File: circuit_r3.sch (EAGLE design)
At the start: 25 parts, among them IC1 7805DT, U1 MCP4725, U2 MB85RC256VPF-G-JNERE2, U4 ATMEGA328P_VQFNVQFN, Y1 16MHz

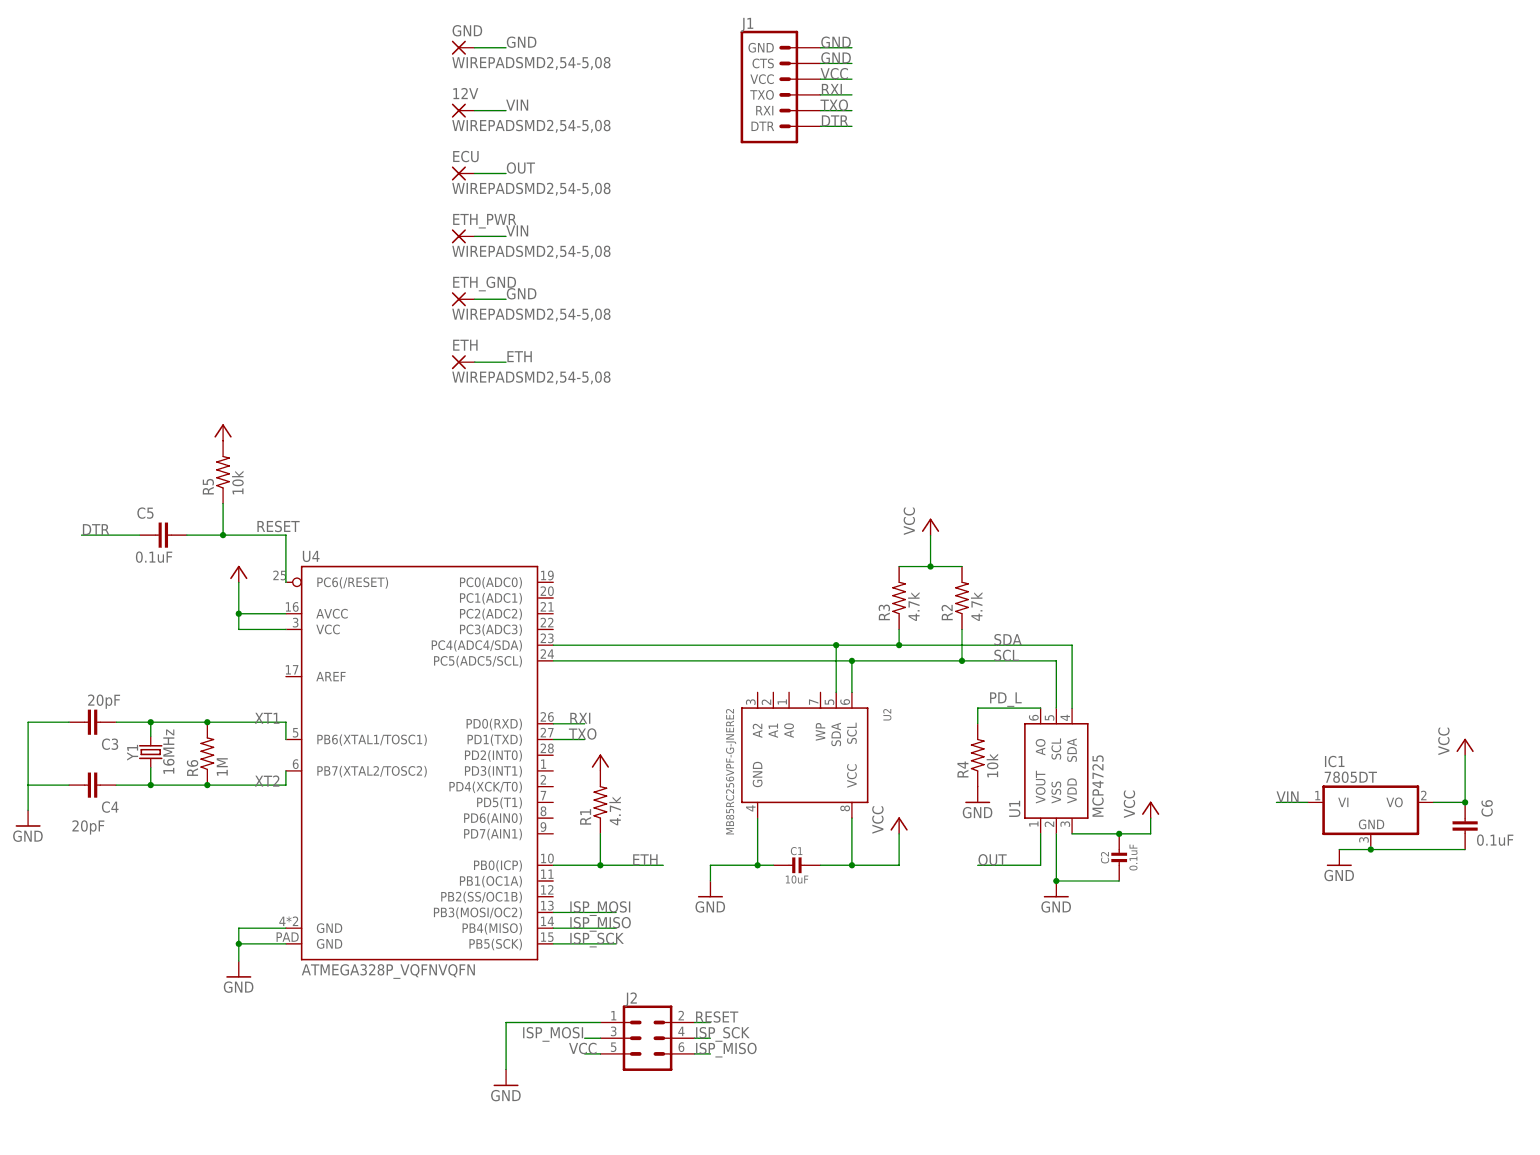
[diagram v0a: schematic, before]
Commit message: Pretty good design.
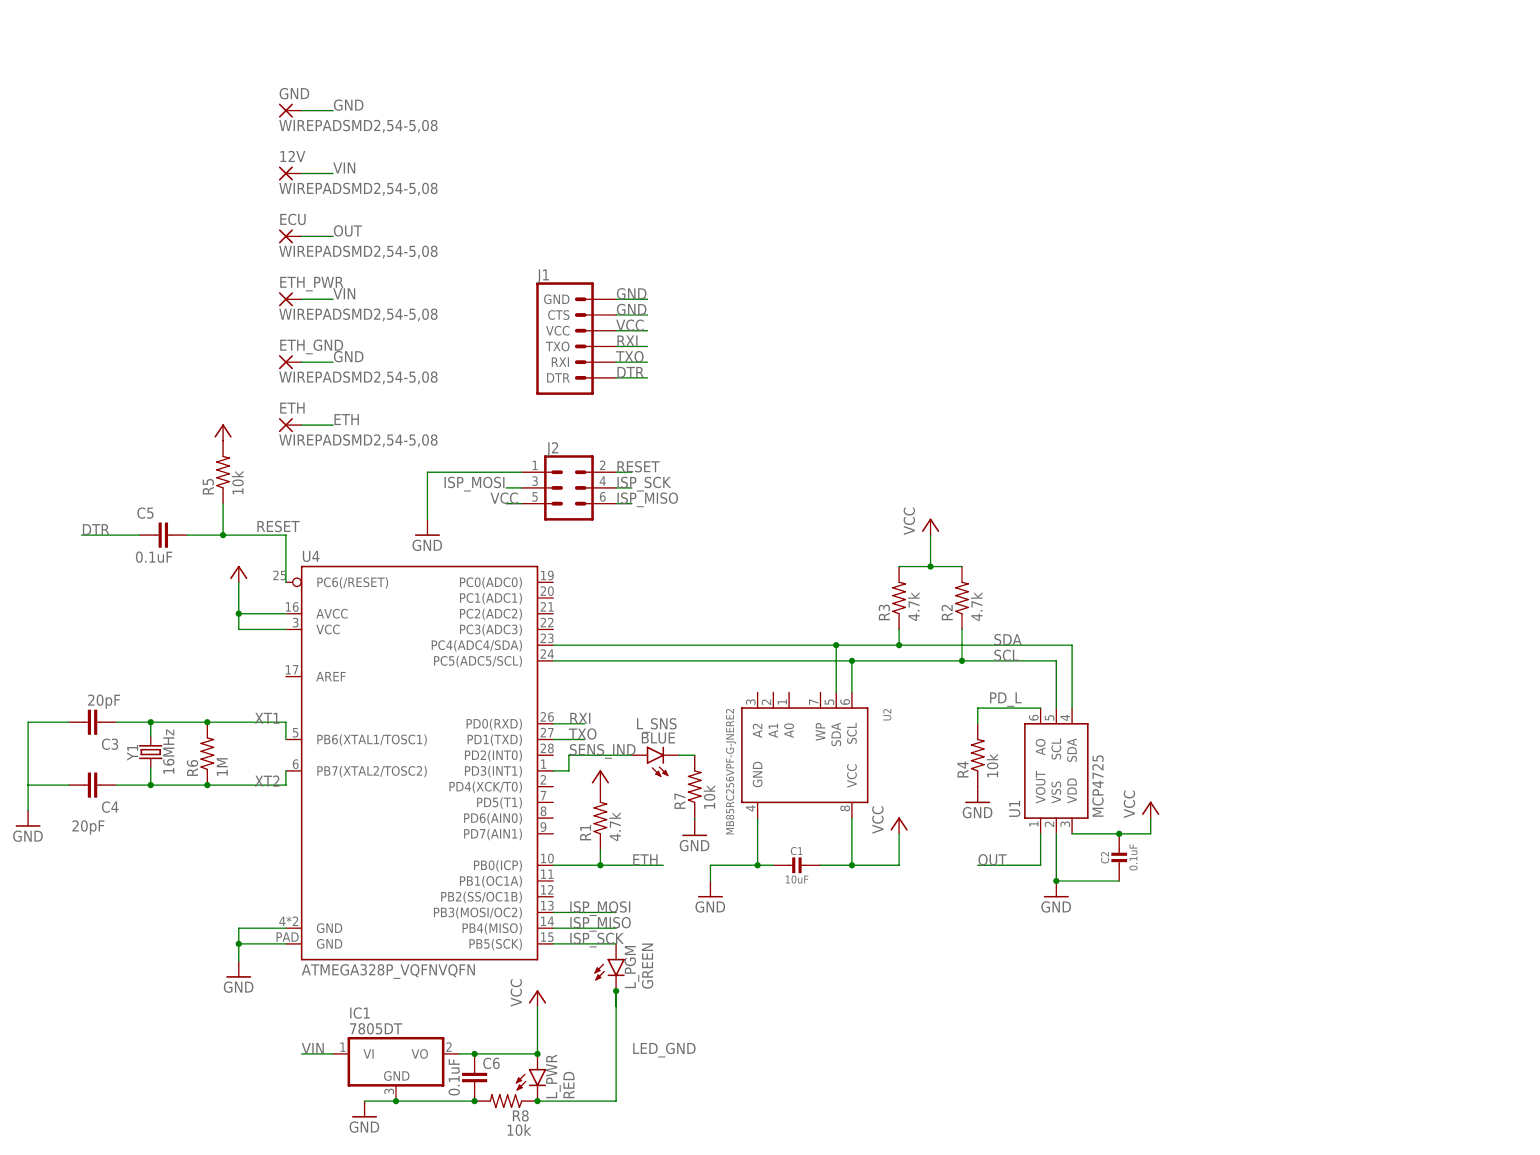
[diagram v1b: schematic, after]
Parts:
- added L_PGM: GREEN, SparkFun-LED:LED-RED0603
- added L_PWR: RED, SparkFun-LED:LED-RED0603
- added L_SNS: BLUE, SparkFun-LED:LED-RED0603
- added R7, R8: 10k, adafruit:R-US_R0603
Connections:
- new net LED_GND: L_PGM.C, L_PWR.C, R8.1
- new net N$2: L_SNS.C, R7.2
- new net SENS_IND: L_SNS.A, U4.PD3(INT1)
- net GND: now also R7.1, R8.2
- net ISP_SCK: now also L_PGM.A
- net VCC: now also L_PWR.A
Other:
- moved on the sheet: 12V, C6, ECU, ETH, ETH_GND, ETH_PWR, GND, IC1, J1, J2, R1
